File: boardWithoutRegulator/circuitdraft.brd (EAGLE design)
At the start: 63 x 37 mm, 36 parts, among them IC1 BQ25887RGER, Q1 16 MHz

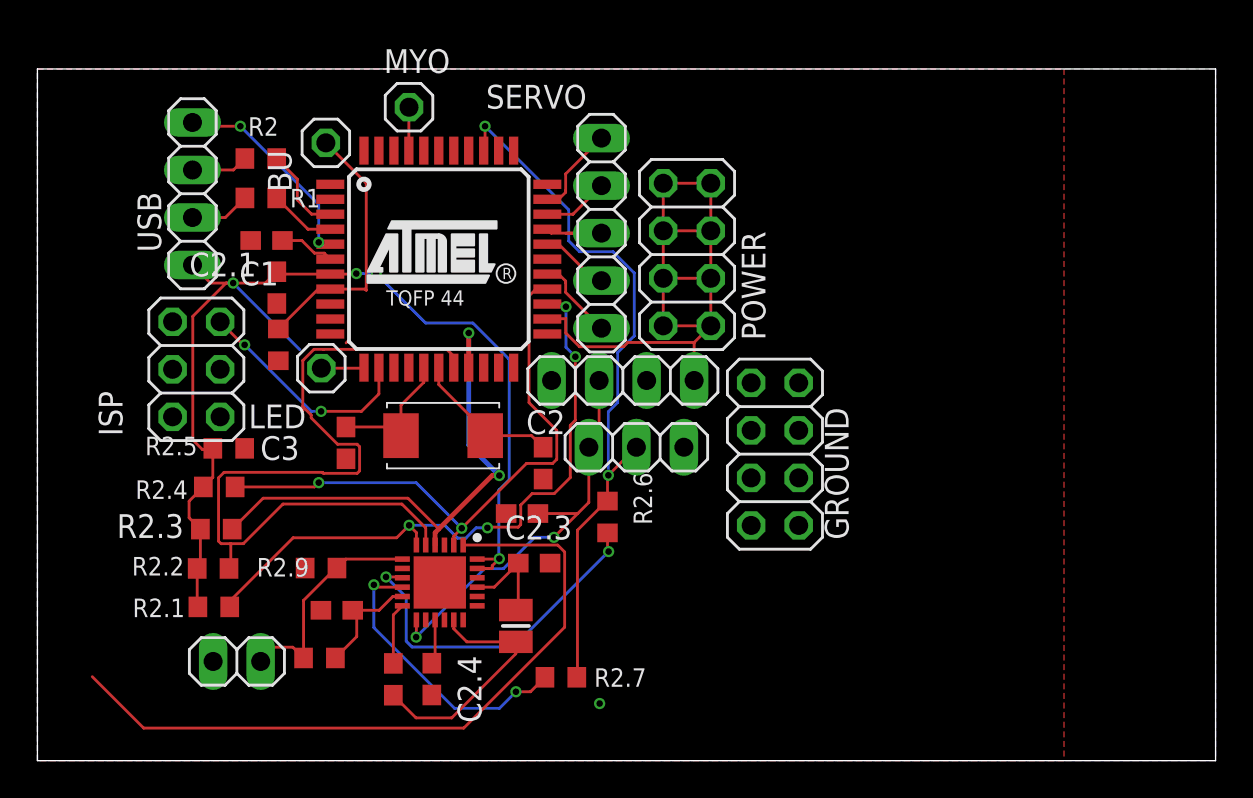
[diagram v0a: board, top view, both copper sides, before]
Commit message: Finished routuing?
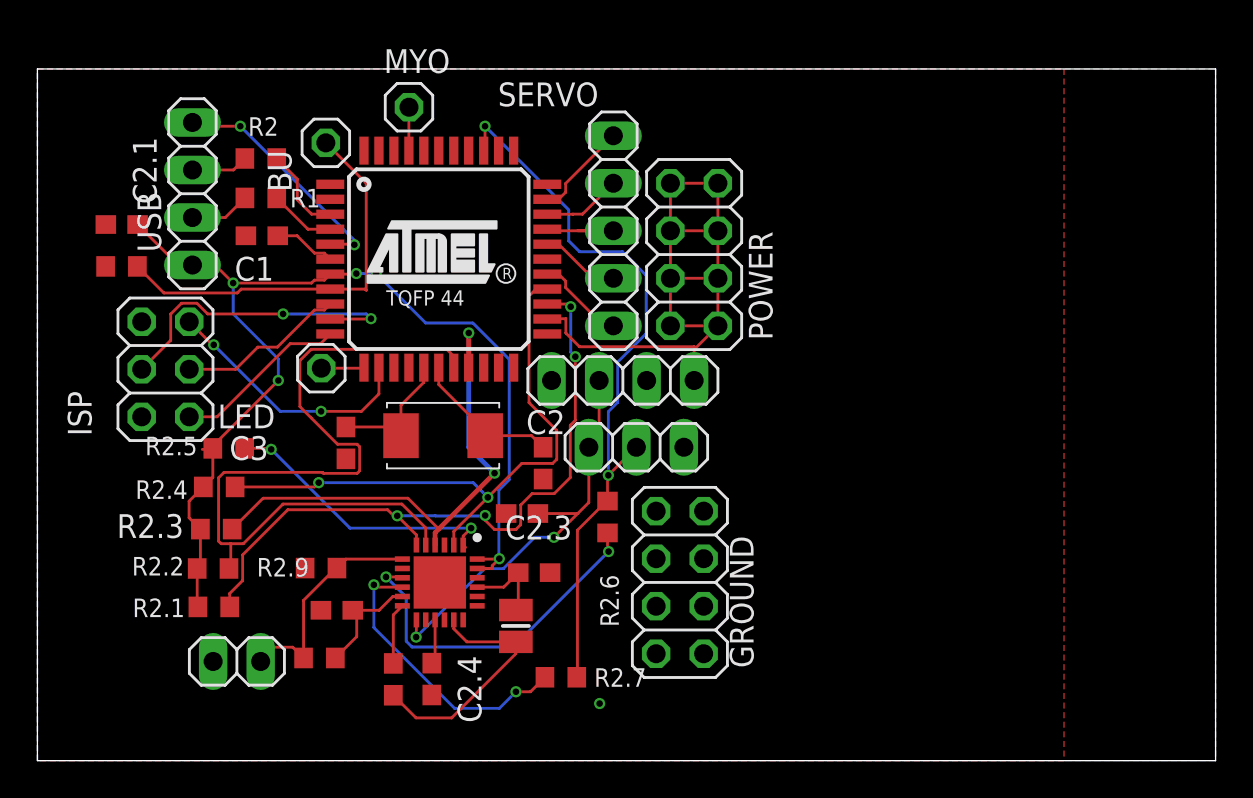
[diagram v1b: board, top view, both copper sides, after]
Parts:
- moved RBUTTON 9.37 mm to (15.5, 26.4), turned to 180 degrees
- moved C2.1 8.95 mm to (15.5, 28.7), turned to 0 degrees
- moved GROUND 8.53 mm to (45.3, 9.53)
- moved ISP 1.65 mm to (17.8, 20.9)
- moved SERVO 0.65 mm to (41.8, 28.3)
- moved C2.6 0.51 mm to (37.6, 10.1)
- moved POWER 0.38 mm to (46.1, 27.1)
- moved C1 0.36 mm to (23.0, 28.1)
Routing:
- net N$7: track 38.6 -> 15.3 mm, vias 0 -> 2
- net MOSI: track 0.00 -> 17.1 mm, vias 0 -> 2
- net MISO: track 0.00 -> 9.37 mm
- net SCK: track 0.00 -> 8.98 mm
- net INTERRUPT: track 14.5 -> 21.8 mm
- net INT: track 34.1 -> 36.9 mm
- net RST: track 12.3 -> 13.9 mm
- net UGND: track 11.4 -> 12.9 mm
- net STAT: track 31.4 -> 32.2 mm
- net MIDDLE: track 38.6 -> 39.4 mm
- net N$21: track 5.29 -> 4.57 mm
- net SIGNAL4: track 3.53 -> 4.22 mm
- net SIGNAL2: track 4.89 -> 5.47 mm
- net SIGNAL1: track 4.21 -> 4.71 mm
- net VBUS: track 58.3 -> 58.0 mm, vias 4 -> 5
